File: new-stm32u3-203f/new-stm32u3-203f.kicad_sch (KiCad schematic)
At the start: 36 parts, among them J1 DM3CS-SF, J2 SJ-3524-SMT, J3 12401826E412A, SW1 SW_SPDT, U1 STM32U385RGT6Q, U2 TLV320DAC3203IRGER, X1 32.768kHz

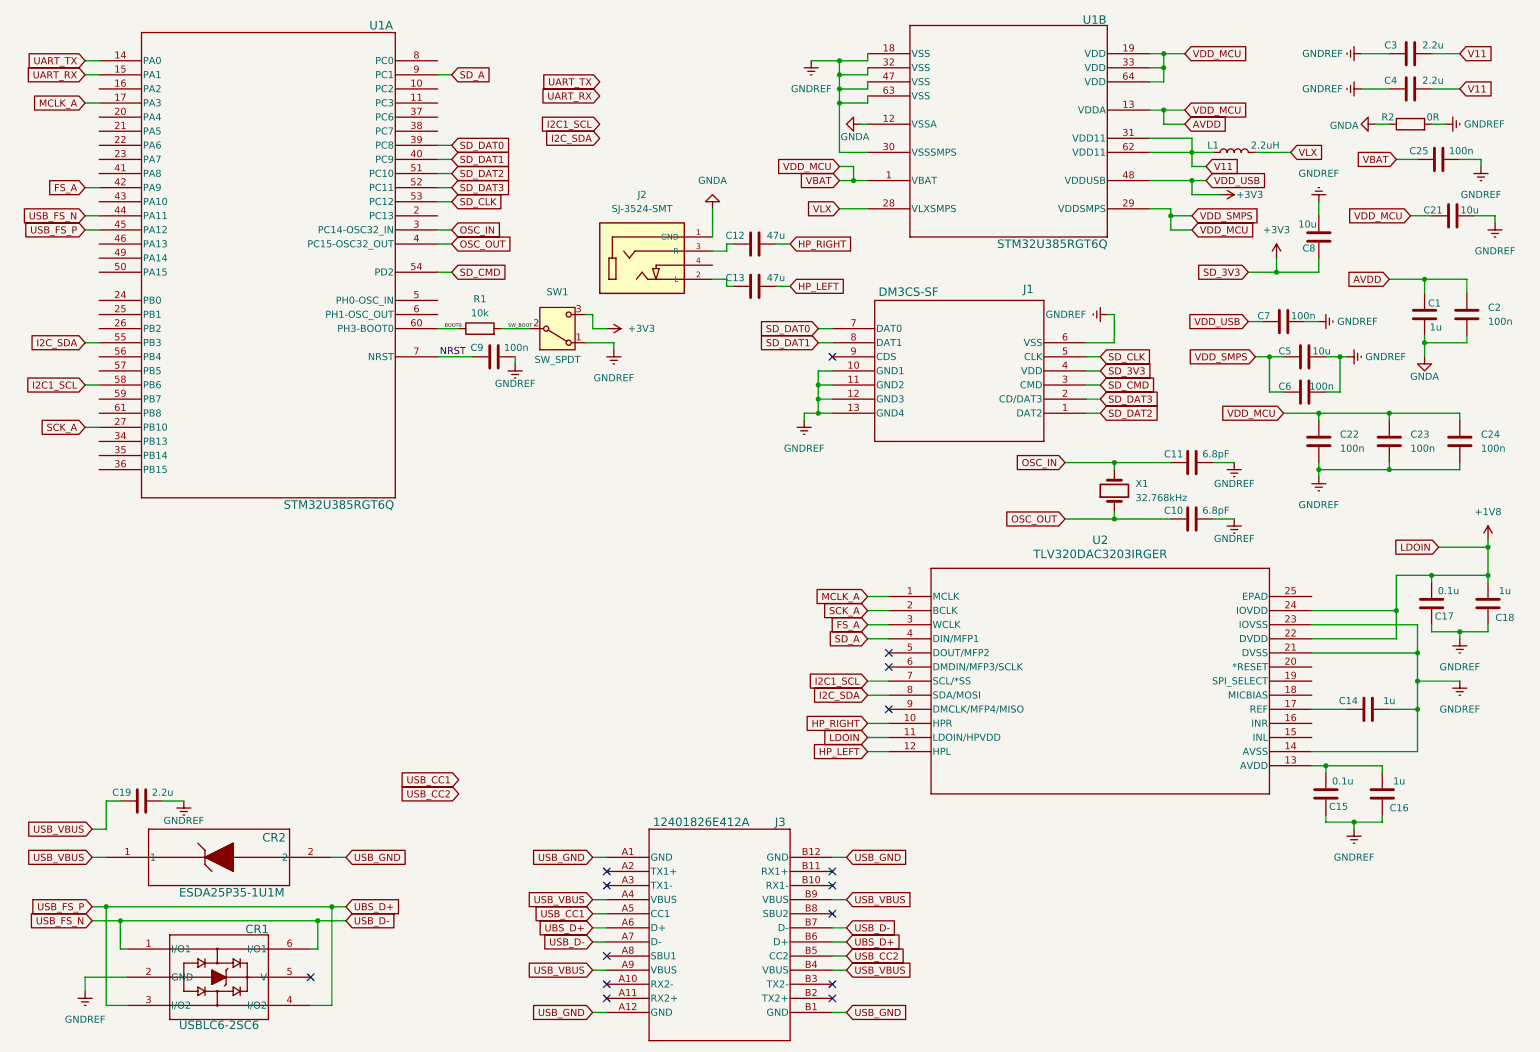
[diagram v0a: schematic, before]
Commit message: made some progress on the board.
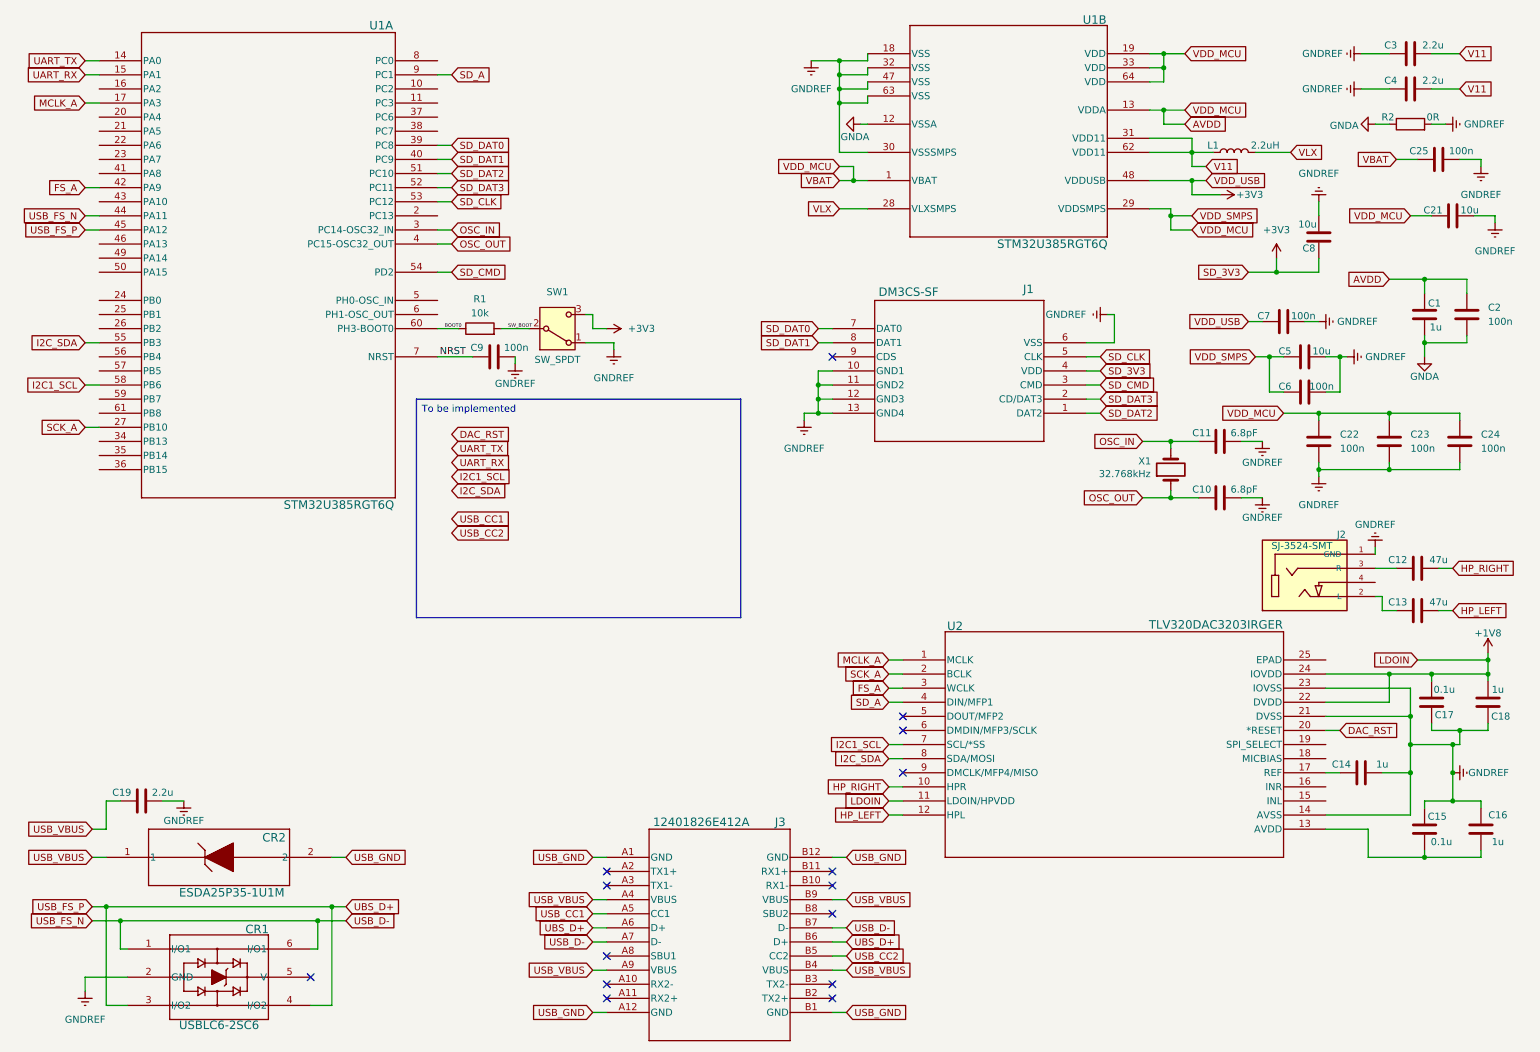
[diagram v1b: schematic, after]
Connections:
- net GNDA: no longer J2.1 (GND)
- net GNDREF: now also J2.1 (GND)
- net DAC_RST: now reaches U2.20 (*RESET)
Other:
- moved on the sheet: C10, C11, C12, C13, C14, C15, C16, C17, C18, J2, U2, X1
